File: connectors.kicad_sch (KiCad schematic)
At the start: 15 parts, among them J1 OLED, J2 SWD, J3 OBDII, SW3 LCD, SW4 MENU

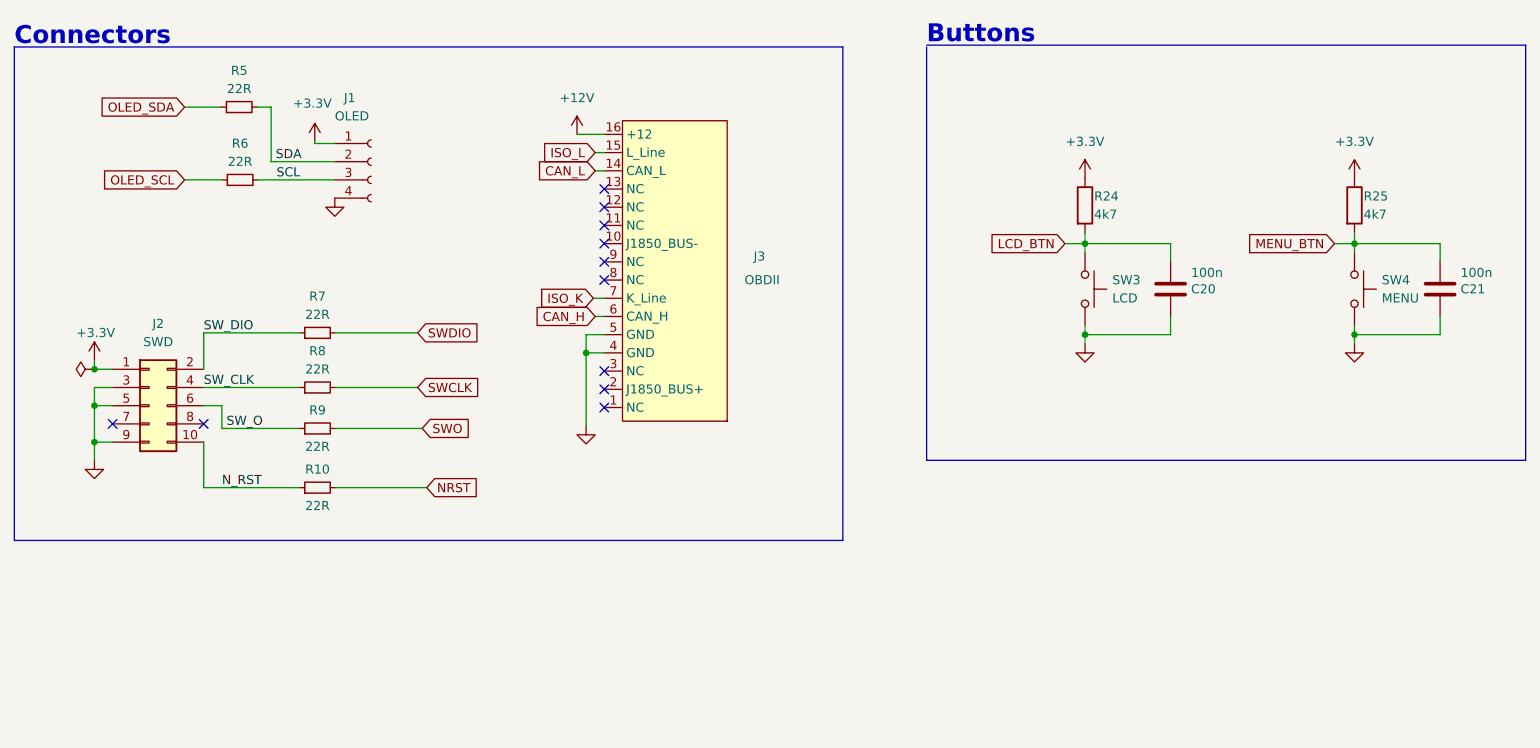
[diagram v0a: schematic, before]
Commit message: KLine update 21/01/23
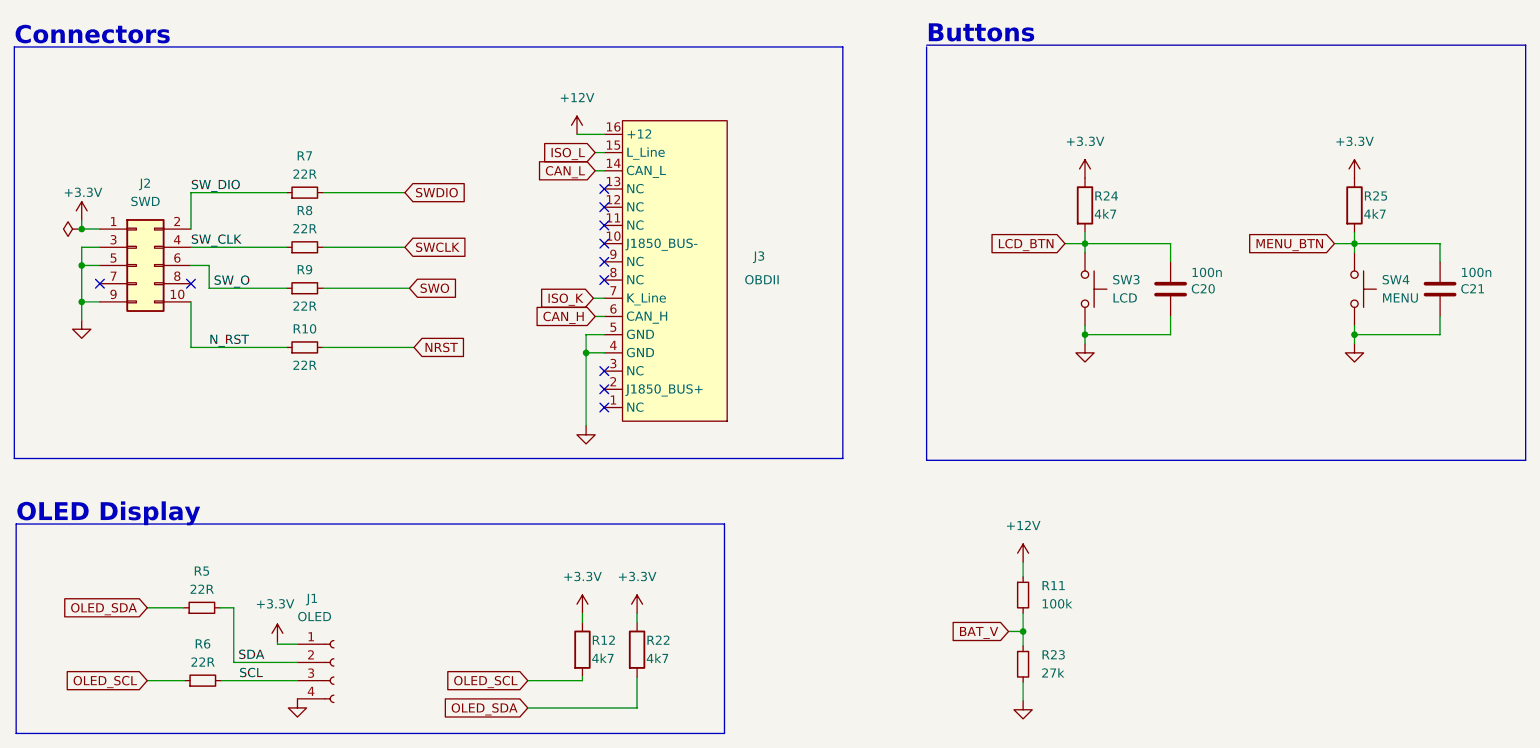
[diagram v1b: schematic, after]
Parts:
- added R11: 100k, Resistor_SMD:R_0402_1005Metric, symbol Device:R_Small
- added R12, R22: 4k7, Resistor_SMD:R_0402_1005Metric, symbol Device:R
- added R23: 27k, Resistor_SMD:R_0402_1005Metric, symbol Device:R_Small
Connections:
- net +12V: now also R11.1
- net +3.3V: now also R12.1, R22.1
- net GND: now also R23.2
- net OLED_SCL: now also R12.2
- net OLED_SDA: now also R22.2
- new net BAT_V: R11.2, R23.1
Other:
- note added: "OLED Display"
- moved on the sheet: J1, J2, R10, R5, R6, R7, R8, R9
